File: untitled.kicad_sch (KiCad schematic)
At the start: 17 parts, among them J1 Conn_02x13_Top_Bottom, J12 Conn_01x03_Pin, J2 Conn_01x13, J3 Conn_02x06_Odd_Even, P1 USB_C_Plug_USB2.0, U5 CP2102N-A02-GQFN28

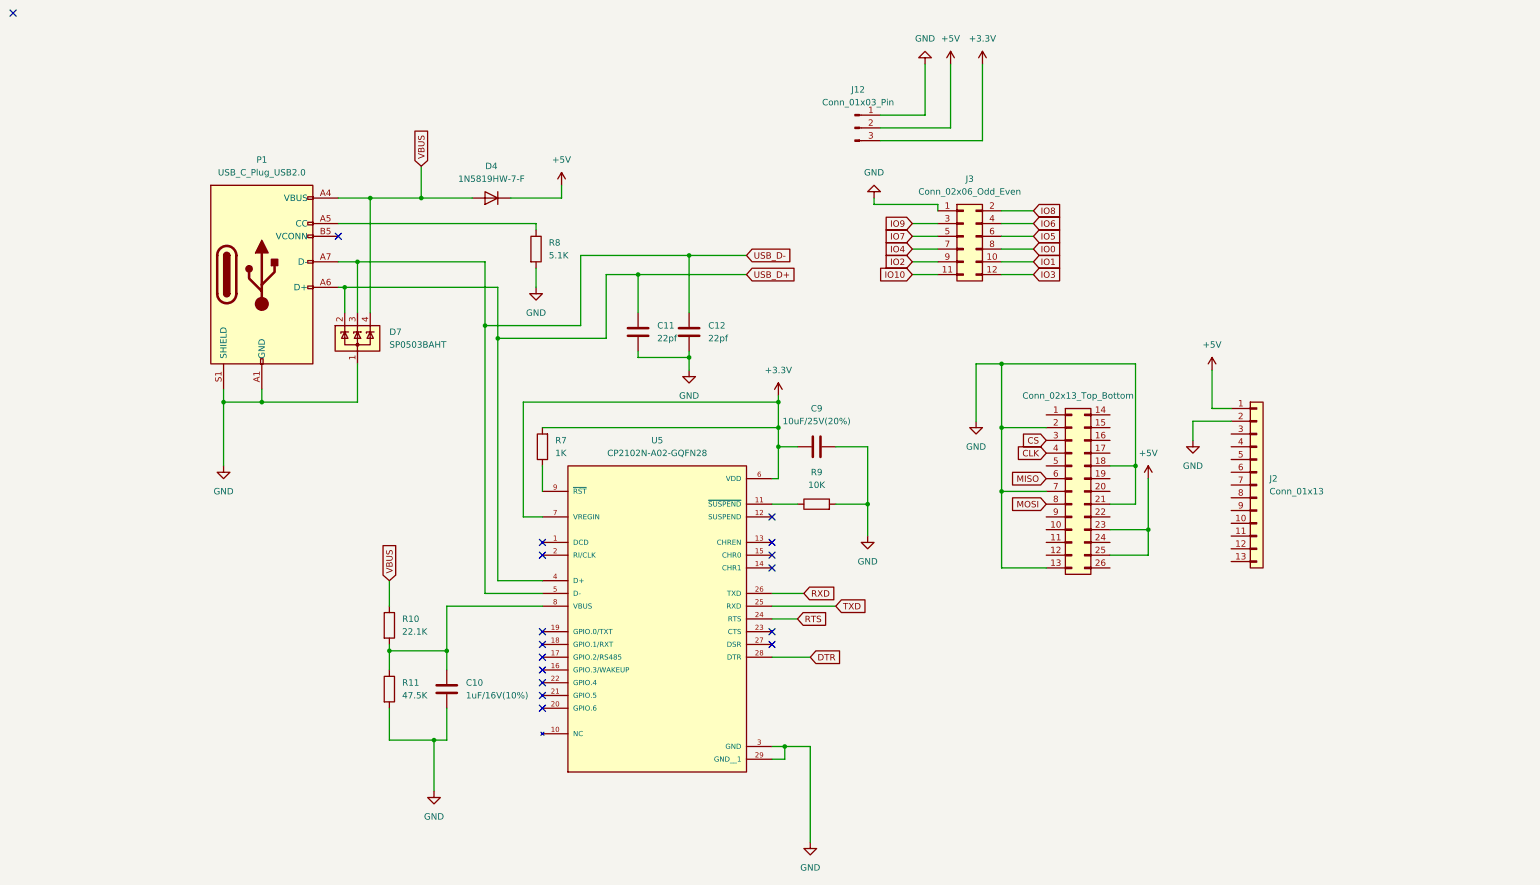
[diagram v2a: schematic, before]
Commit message: Update to v3.1
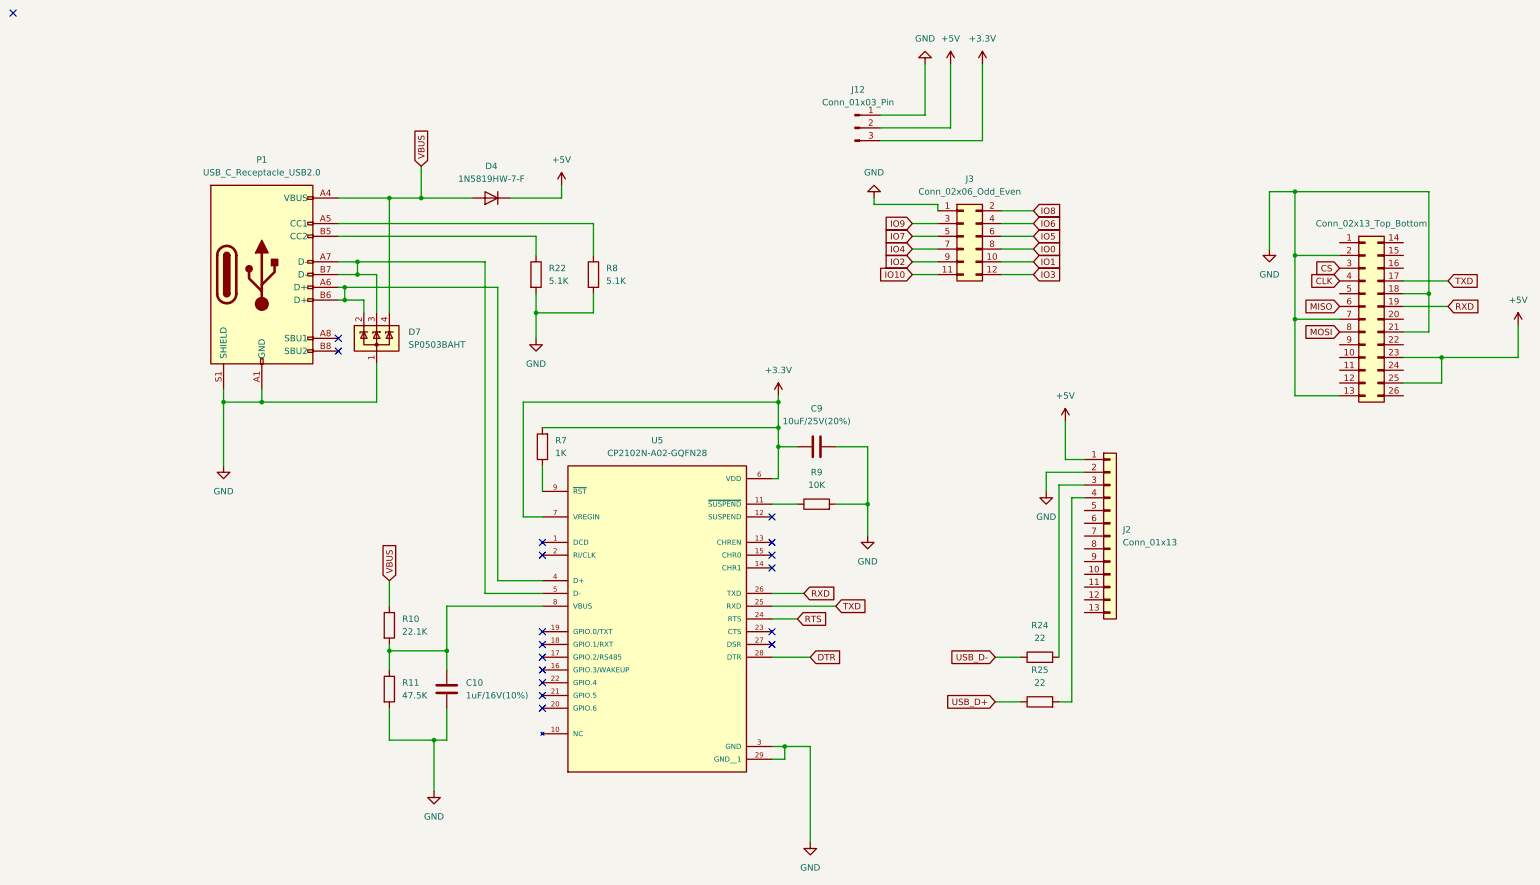
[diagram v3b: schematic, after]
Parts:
- removed C11, C12: 22pf, Capacitor_SMD:C_0603_1608Metric, symbol Device:C
- added R22: 5.1K, Resistor_SMD:R_0603_1608Metric, symbol Device:R
- added R24, R25: 22, Resistor_SMD:R_0603_1608Metric, symbol Device:R
- C10, C9: footprint Capacitor_SMD:C_0402_1005Metric -> Capacitor_SMD:C_0603_1608Metric
- P1: value USB_C_Plug_USB2.0 -> USB_C_Receptacle_USB2.0; symbol Connector:USB_C_Plug_USB2.0 -> Connector:USB_C_Receptacle_USB2.0
- R10, R11, R7, R9: footprint Resistor_SMD:R_0402_1005Metric -> Resistor_SMD:R_0603_1608Metric
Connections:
- net GND: now also R22.2
- net RXD: now also J1.19 (Pin_19)
- net TXD: now also J1.17 (Pin_17)
- net USB_D+: now also R25.1; no longer D7.2 (K), P1.A6 (D+), U5.4 (D+)
- net USB_D-: now also R24.1; no longer D7.3 (K), P1.A7 (D-), U5.5 (D-)
- net at J2.3 (Pin_3): now also R24.2
- net at J2.4 (Pin_4): now also R25.2
- net at P1.B5 (CC2): now also R22.1
- new net: D7.2 (K), P1.A6 (D+), P1.B6 (D+), U5.4 (D+)
- new net: D7.3 (K), P1.A7 (D-), P1.B7 (D-), U5.5 (D-)
- no-connect marks 17 -> 18
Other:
- moved on the sheet: D7, J2, R8
